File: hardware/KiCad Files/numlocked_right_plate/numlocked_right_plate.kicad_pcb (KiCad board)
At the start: 2 copper layers, 207.1 x 143.2 mm, 6 parts

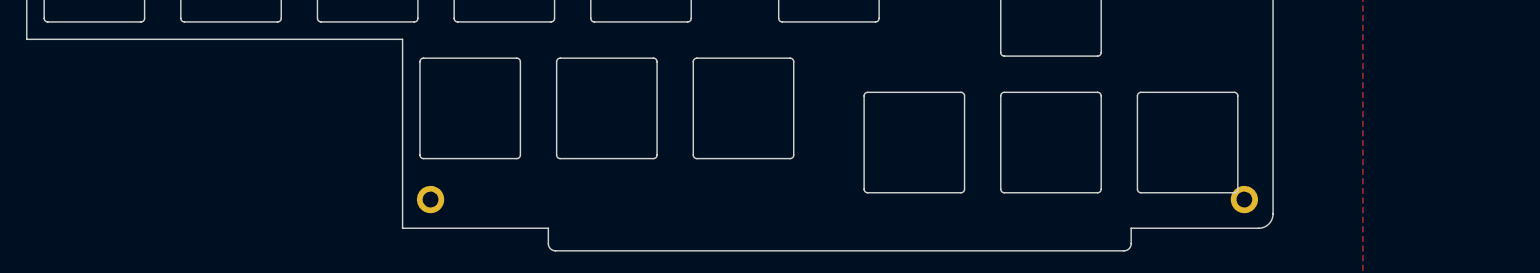
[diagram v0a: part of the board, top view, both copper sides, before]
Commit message: Another quick hardware push. Sorry Github servers.
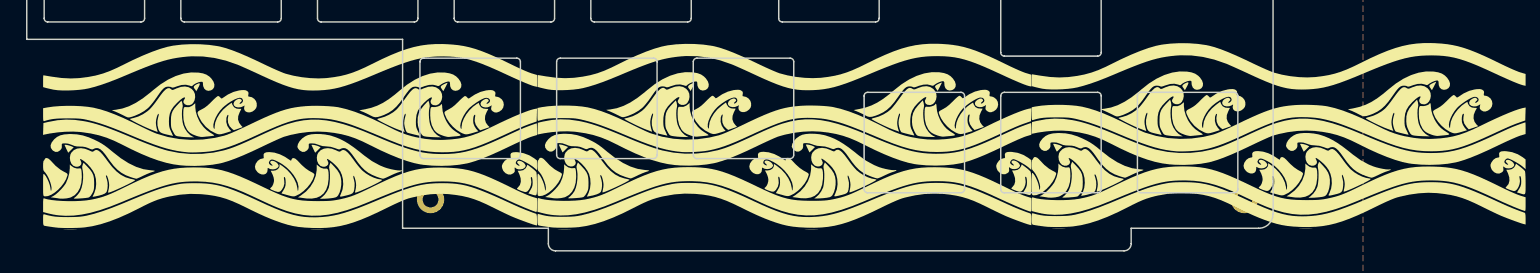
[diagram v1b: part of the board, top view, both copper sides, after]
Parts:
- added G***: LOGO, LOGO, F.Cu at (267.9, 152.1)
- added G***: LOGO, LOGO, F.Cu at (130.0, 152.2)
- added G***: LOGO, LOGO, F.Cu at (198.9, 152.2)
